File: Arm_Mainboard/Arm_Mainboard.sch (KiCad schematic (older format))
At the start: 31 parts

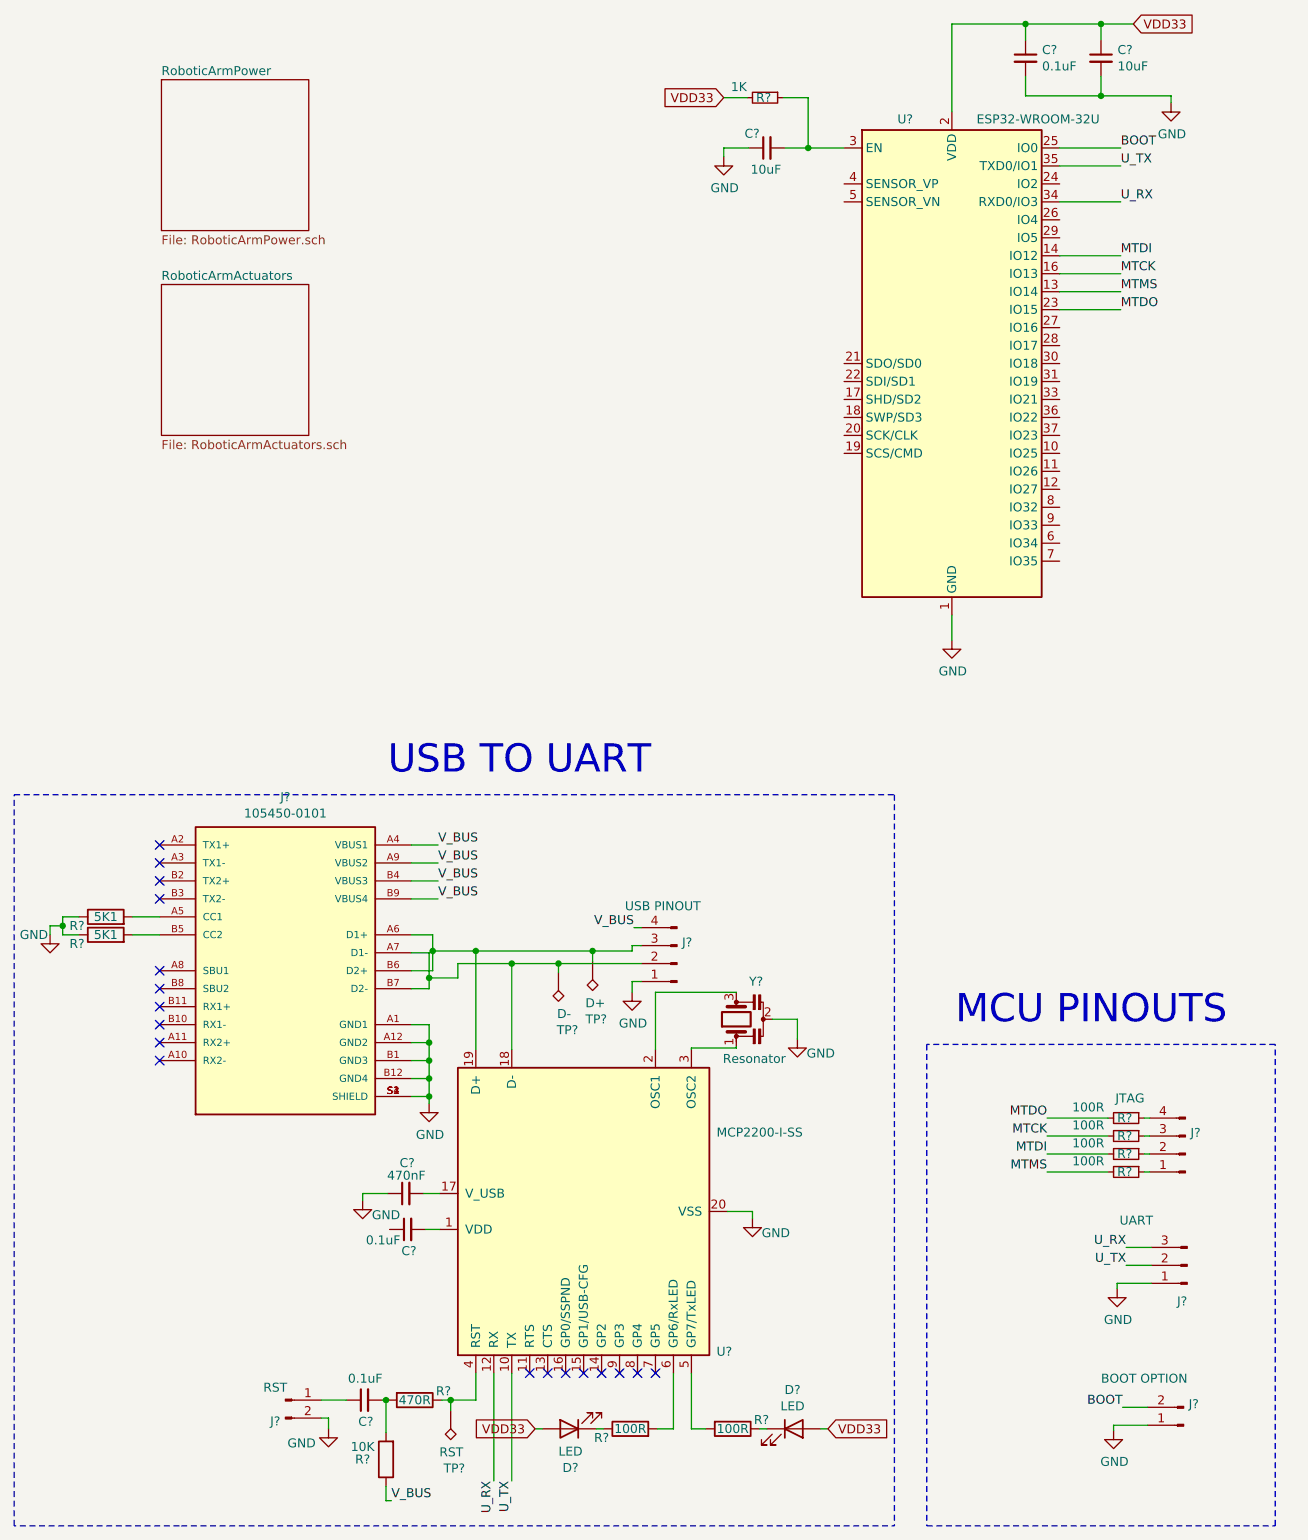
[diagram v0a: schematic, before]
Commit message: PCB
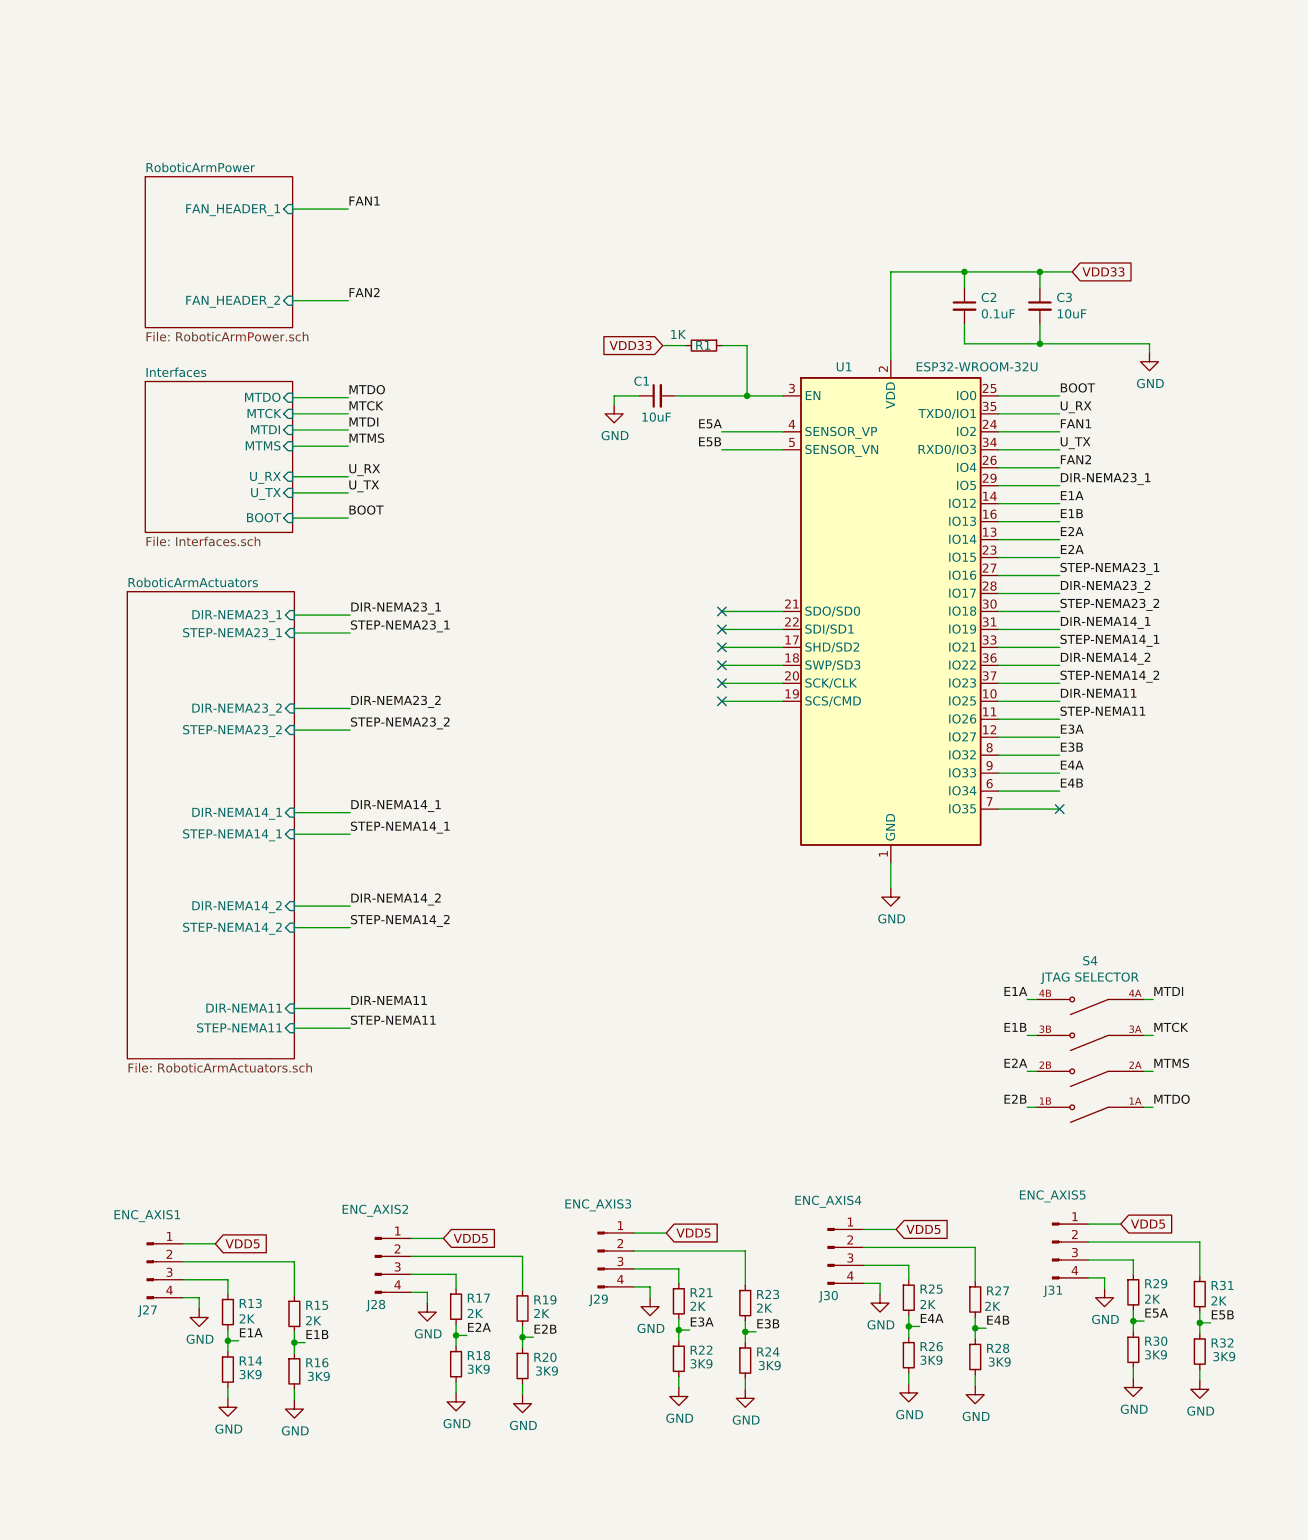
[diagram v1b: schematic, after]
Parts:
- removed C?: 470nF, symbol Device:C_Small
- removed C? (x2): 0.1uF, symbol Device:C_Small
- removed D? (x2): LED, Diode_SMD:D_1206_3216Metric_Castellated, symbol Device:LED
- removed J?: UART, Connector_PinSocket_2.54mm:PinSocket_1x03_P2.54mm_Vertical, symbol Connector:Conn_01x03_Male
- removed J?: JTAG, Connector_PinSocket_2.54mm:PinSocket_1x04_P2.54mm_Vertical, symbol Connector:Conn_01x04_Male
- removed J?: BOOT OPTION, Jumper:SolderJumper-2_P1.3mm_Open_RoundedPad1.0x1.5mm, symbol Connector:Conn_01x02_Male
- removed J?: USB PINOUT, symbol Connector:Conn_01x04_Male
- removed J?: RST, Jumper:SolderJumper-2_P1.3mm_Open_RoundedPad1.0x1.5mm, symbol Connector:Conn_01x02_Male
- removed J?: 105450-0101, MOLEX_105450-0101, symbol 105450-0101:105450-0101
- removed R? (x4): 100R, symbol Device:R_Small
- removed R?: 470R, symbol Device:R
- removed R?: 10K, symbol Device:R
- removed R? (x2): 100R, symbol Device:R
- removed R? (x2): 5K1, symbol Device:R
- removed TP?: D-, symbol Connector:TestPoint_Alt
- removed TP?: D+, symbol Connector:TestPoint_Alt
- removed TP?: RST, symbol Connector:TestPoint_Alt
- removed U?: MCP2200-I-SS, Package_SO:SSOP-20_5.3x7.2mm_P0.65mm, symbol Interface_USB:MCP2200-I-SS
- removed Y?: Resonator, Crystal:Resonator_SMD_muRata_CSTxExxV-3Pin_3.0x1.1mm, symbol Device:Resonator
- added J27: ENC_AXIS1, Connector_JST:JST_EH_S4B-EH_1x04_P2.50mm_Horizontal, symbol Connector:Conn_01x04_Male
- added J28: ENC_AXIS2, Connector_JST:JST_EH_S4B-EH_1x04_P2.50mm_Horizontal, symbol Connector:Conn_01x04_Male
- added J29: ENC_AXIS3, Connector_JST:JST_EH_S4B-EH_1x04_P2.50mm_Horizontal, symbol Connector:Conn_01x04_Male
- added J30: ENC_AXIS4, Connector_JST:JST_EH_S4B-EH_1x04_P2.50mm_Horizontal, symbol Connector:Conn_01x04_Male
- added J31: ENC_AXIS5, Connector_JST:JST_EH_S4B-EH_1x04_P2.50mm_Horizontal, symbol Connector:Conn_01x04_Male
- added R13, R15, R17, R19, R21, R23, R25, R27, R29, R31: 2K, Resistor_SMD:R_0805_2012Metric_Pad1.20x1.40mm_HandSolder, symbol Device:R_Small
- added R14, R16, R18, R20, R22, R24, R26, R28, R30, R32: 3K9, Resistor_SMD:R_0805_2012Metric_Pad1.20x1.40mm_HandSolder, symbol Device:R_Small
- added S4: JTAG SELECTOR, ArmFootprints:SW_DS04-254-2-04BK-SMT, symbol DS04-254-2-04BK-SMT:DS04-254-2-04BK-SMT
- C1, C2, C3: renamed from C?; footprint (none) -> Capacitor_SMD:C_0805_2012Metric_Pad1.18x1.45mm_HandSolder
- R1: renamed from R?; footprint (none) -> Resistor_SMD:R_0805_2012Metric_Pad1.20x1.40mm_HandSolder
- gave numbers to parts that had none: 1
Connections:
- net GND: now also J27.4 (Pin_4), J28.4 (Pin_4), J29.4 (Pin_4), J30.4 (Pin_4), J31.4 (Pin_4), R14.2, R16.2, R18.2, R20.2, R22.2, R24.2, R26.2, R28.2, R30.2, R32.2
- net MTCK: now also S4.3A; no longer U1.16 (IO13)
- net MTDI: now also S4.4A; no longer U1.14 (IO12)
- net MTDO: now also S4.1A; no longer U1.23 (IO15)
- net MTMS: now also S4.2A; no longer U1.13 (IO14)
- net U_RX: now also U1.35 (TXD0/IO1); no longer U1.34 (RXD0/IO3)
- net U_TX: now also U1.34 (RXD0/IO3); no longer U1.35 (TXD0/IO1)
- net DIR-NEMA11: now reaches U1.10 (IO25)
- net STEP-NEMA11: now reaches U1.11 (IO26)
- net E3A: now reaches U1.12 (IO27)
- net E3A: now also R21.2, R22.1
- net FAN1: now reaches U1.24 (IO2)
- net FAN2: now reaches U1.26 (IO4)
- net STEP-NEMA23_1: now reaches U1.27 (IO16)
- net DIR-NEMA23_2: now reaches U1.28 (IO17)
- net DIR-NEMA23_1: now reaches U1.29 (IO5)
- net STEP-NEMA23_2: now reaches U1.30 (IO18)
- net DIR-NEMA14_1: now reaches U1.31 (IO19)
- net STEP-NEMA14_1: now reaches U1.33 (IO21)
- net DIR-NEMA14_2: now reaches U1.36 (IO22)
- net STEP-NEMA14_2: now reaches U1.37 (IO23)
- net E5A: now reaches U1.4 (SENSOR_VP)
- net E5A: now also R29.2, R30.1
- net E5B: now reaches U1.5 (SENSOR_VN)
- net E5B: now also R31.2, R32.1
- net E4B: now reaches U1.6 (IO34)
- net E4B: now also R27.2, R28.1
- net E3B: now reaches U1.8 (IO32)
- net E3B: now also R23.2, R24.1
- net E4A: now reaches U1.9 (IO33)
- net E4A: now also R25.2, R26.1
- new net: J27.2 (Pin_2), R15.1
- new net: J27.3 (Pin_3), R13.1
- new net: J28.2 (Pin_2), R19.1
- new net: J28.3 (Pin_3), R17.1
- new net: J29.2 (Pin_2), R23.1
- new net: J29.3 (Pin_3), R21.1
- new net: J30.2 (Pin_2), R27.1
- new net: J30.3 (Pin_3), R25.1
- new net: J31.2 (Pin_2), R31.1
- new net: J31.3 (Pin_3), R29.1
- new net E1A: R13.2, R14.1, S4.4B, U1.14 (IO12)
- new net E1B: R15.2, R16.1, S4.3B, U1.16 (IO13)
- new net E2A: R17.2, R18.1, S4.2B, U1.13 (IO14), U1.23 (IO15)
- new net E2B: R19.2, R20.1, S4.1B
- new net VDD5: J27.1 (Pin_1), J28.1 (Pin_1), J29.1 (Pin_1), J30.1 (Pin_1), J31.1 (Pin_1)
- no-connect marks 18 -> 7
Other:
- note removed: "MCU PINOUTS\n"
- note removed: "USB TO UART"
- moved on the sheet: C1, C2, C3, R1, U1
